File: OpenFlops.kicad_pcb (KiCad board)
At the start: 2 copper layers, 112 x 59 mm, 66 parts, among them J7 DISPLAY_PORT, P1 FLOPPY_CONN, P2 POWER_INPUT, P3 USB_A_FEMALE, P4 PROG_PORT, P5 JUMPERS, Q1 MOS_N_GSD, Q2 MOS_N_GSD, Q3 MOS_N_GSD, Q4 MOS_N_GSD, Q5 MOS_N_GSD, Q6 MOS_N_GSD, U1 74HC04, U3 STM32F105RBT6, U4 LM1117-3.3, U8 W25Q32JVSS (?), Y1 8 MHz

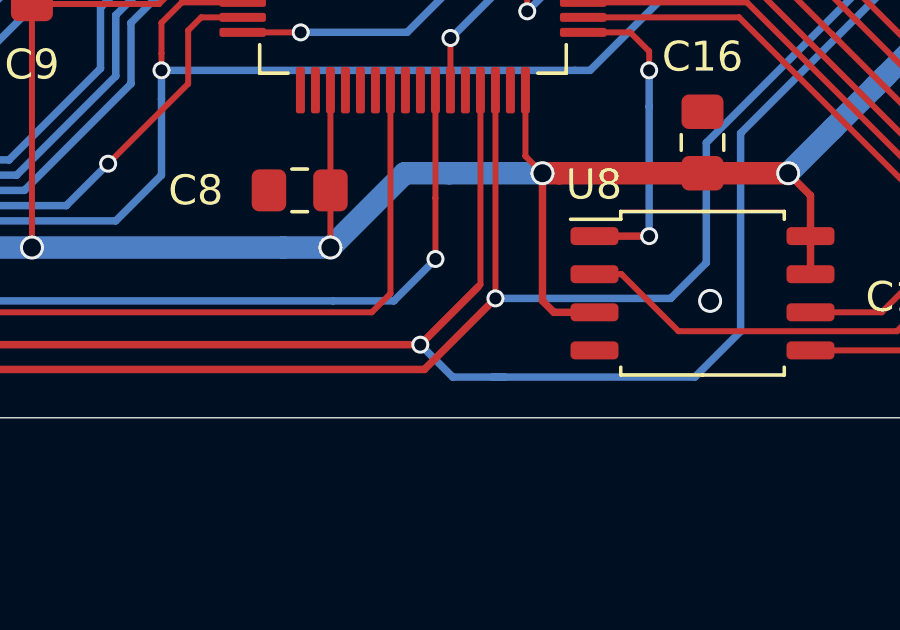
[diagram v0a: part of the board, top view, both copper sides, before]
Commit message: Fix track width
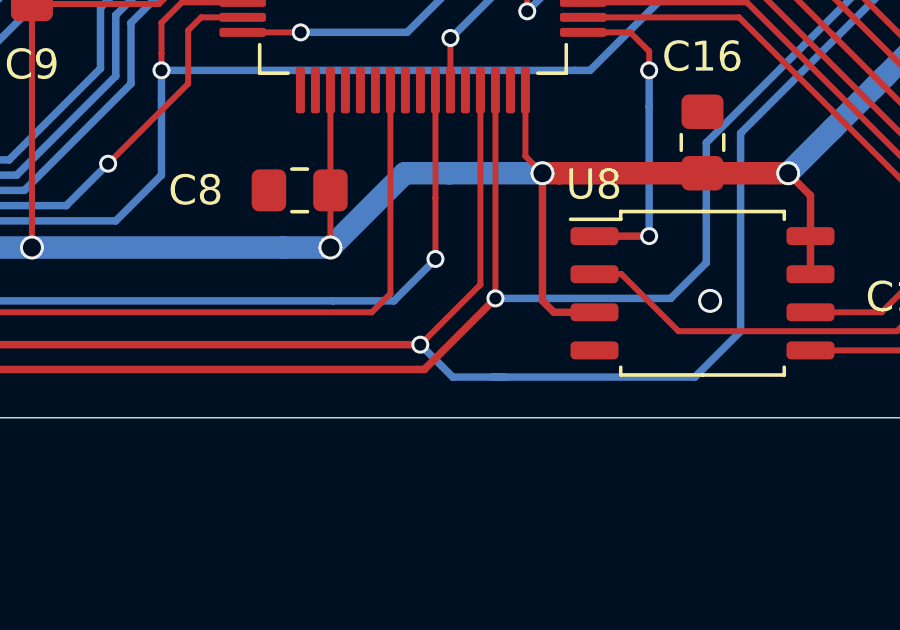
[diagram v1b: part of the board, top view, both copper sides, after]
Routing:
- net /disp_dio: track 81.8 -> 79.7 mm
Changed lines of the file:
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@@
     (thickness 1.6)
     (drawings 24)
-    (tracks 766)
+    (tracks 764)
     (zones 0)
     (modules 66)
@@
   (segment (start 195.199 69.024499) (end 195.135501 69.024499) (width 0.25) (layer B.Cu) (net 12))
   (segment (start 169.89 83.907) (end 169.89 90.388) (width 0.2) (layer F.Cu) (net 12))
-  (segment (start 167.8855 92.3925) (end 169.8265 90.4515) (width 0.25) (layer F.Cu) (net 12))
-  (segment (start 169.8265 90.4515) (end 168.33 91.948) (width 0.2) (layer F.Cu) (net 12))
-  (segment (start 169.89 90.388) (end 169.8265 90.4515) (width 0.2) (layer F.Cu) (net 12))
   (via (at 167.8855 92.3925) (size 0.6) (drill 0.4) (layers F.Cu B.Cu) (net 12))
   (segment (start 168.965 93.472) (end 170.688 93.472) (width 0.25) (layer B.Cu) (net 12))
@@
   (segment (start 148.59 98.230081) (end 148.59 93.98) (width 0.25) (layer F.Cu) (net 12))
   (segment (start 146.812 98.806) (end 148.014081 98.806) (width 0.25) (layer F.Cu) (net 12))
+  (segment (start 169.89 90.388) (end 167.8855 92.3925) (width 0.2) (layer F.Cu) (net 12))
   (via (at 125.6665 97.282) (size 0.6) (drill 0.4) (layers F.Cu B.Cu) (net 13))
   (via (at 113.157 94.615) (size 0.6) (drill 0.4) (layers F.Cu B.Cu) (net 13))
@@
     (connect_pads (clearance 0.254))
     (min_thickness 0.0254)
-    (fill yes (arc_segments 32) (thermal_gap 0.508) (thermal_bridge_width 0.508))
+    (fill (arc_segments 32) (thermal_gap 0.508) (thermal_bridge_width 0.508))
     (polygon
       (pts
@@
     (connect_pads (clearance 0.254))
     (min_thickness 0.0254)
-    (fill yes (arc_segments 32) (thermal_gap 0.508) (thermal_bridge_width 0.508))
+    (fill (arc_segments 32) (thermal_gap 0.508) (thermal_bridge_width 0.508))
     (polygon
       (pts
